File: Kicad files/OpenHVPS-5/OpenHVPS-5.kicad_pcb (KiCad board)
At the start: 2 copper layers, 40.6 x 20.8 mm, 84 parts, among them J1 Conn_01x03_Male, Q1 FQT7N10, Q2 BC846A, Q3 MMBT3906, Q4 MMBT3906, U1 MAX6008AEUR+T, U2 74HC14, U3 MAX4162, U4 CD14538BM

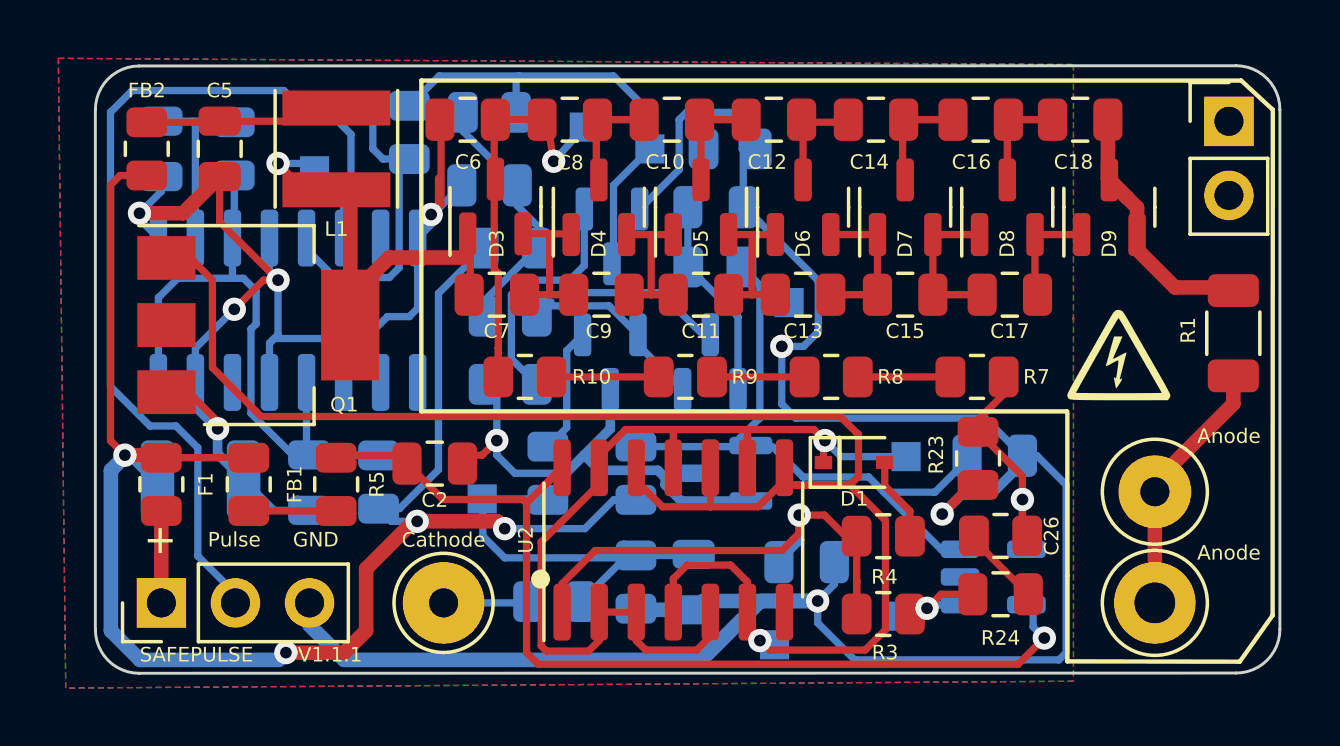
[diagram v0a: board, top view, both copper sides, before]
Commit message: Updated  with TP and some other small changes.
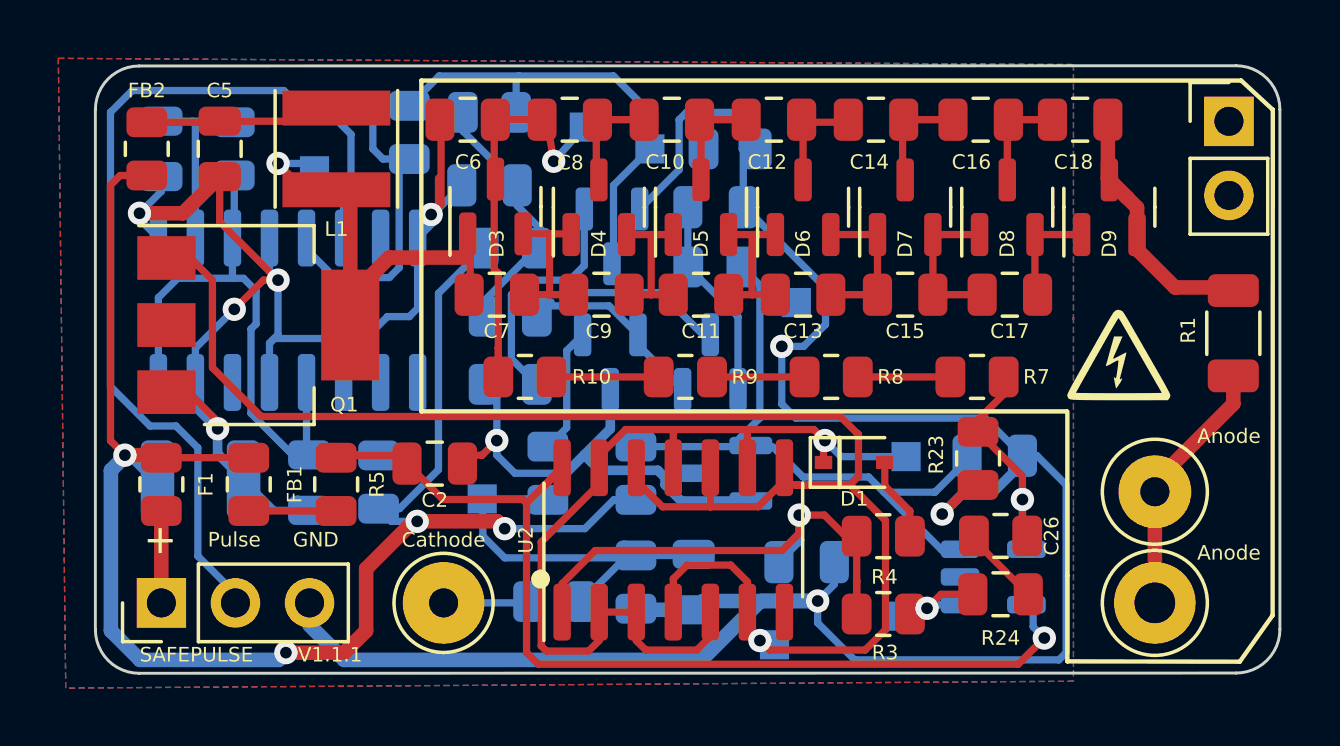
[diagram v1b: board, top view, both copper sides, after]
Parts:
- moved TP1 0.25 mm to (150.3, 65.3)
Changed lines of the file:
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@@
   )
   (footprint "TestPoint:TestPoint_Pad_1.0x1.0mm" (layer "B.Cu")
-    (at 150.02 65.27 180)
+    (at 150.27 65.27 180)
     (descr "SMD rectangular pad as test Point, square 1.0mm side length")
     (tags "test point SMD pad rectangle square")
@@
   (segment (start 142.433 71.12) (end 140.62 71.12) (width 0.25) (layer "B.Cu") (net 3))
   (segment (start 127.75 62.208) (end 127.75 62.41) (width 0.25) (layer "B.Cu") (net 3))
+  (segment (start 148.45 62) (end 148.5 62) (width 0.25) (layer "B.Cu") (net 3))
   (segment (start 152.27 77.52) (end 159.27 77.52) (width 0.25) (layer "B.Cu") (net 3))
-  (segment (start 148.45 62) (end 148.5 62) (width 0.25) (layer "B.Cu") (net 3))
   (segment (start 134.1026 66.5) (end 134.747 67.1444) (width 0.25) (layer "B.Cu") (net 3))
   (segment (start 127.75 62.41) (end 128.397 63.057) (width 0.25) (layer "B.Cu") (net 3))
   (segment (start 139.428 68.072) (end 139.5495 68.072) (width 0.25) (layer "B.Cu") (net 3))
+  (segment (start 151.27 64.77) (end 151.27 66.02) (width 0.25) (layer "B.Cu") (net 3))
   (segment (start 137.832 62.332) (end 137.832 62.5121) (width 0.25) (layer "B.Cu") (net 3))
   (segment (start 149.77 68.75) (end 150.25 69.23) (width 0.25) (layer "B.Cu") (net 3))
@@
   (segment (start 137.75 62.25) (end 137.8 62.25) (width 0.25) (layer "B.Cu") (net 3))
   (segment (start 151 76.25) (end 152.27 77.52) (width 0.25) (layer "B.Cu") (net 3))
+  (segment (start 150.52 66.77) (end 149.77 66.77) (width 0.25) (layer "B.Cu") (net 3))
   (segment (start 148.4125 59.1625) (end 148.4125 60) (width 0.25) (layer "B.Cu") (net 3))
   (segment (start 149.04 75.5) (end 151 75.5) (width 0.5) (layer "B.Cu") (net 3))
@@
   (segment (start 148.336 72.0325) (end 148.37 72.0665) (width 0.25) (layer "B.Cu") (net 3))
   (segment (start 158.02 70.77) (end 158.02 70.52) (width 0.3302) (layer "B.Cu") (net 3))
-  (segment (start 151.02 64.52) (end 151.02 66.27) (width 0.25) (layer "B.Cu") (net 3))
   (segment (start 132.5 64.5) (end 132.5 66.3677) (width 0.25) (layer "B.Cu") (net 3))
   (segment (start 151 75.5) (end 151 76.25) (width 0.25) (layer "B.Cu") (net 3))
@@
   (segment (start 128.5 61.458) (end 128.5 60.95) (width 0.25) (layer "B.Cu") (net 3))
   (segment (start 142.993864 70.493864) (end 143.52 71.02) (width 0.3302) (layer "B.Cu") (net 3))
-  (segment (start 150.52 66.77) (end 149.77 66.77) (width 0.25) (layer "B.Cu") (net 3))
   (segment (start 159.27 77.52) (end 159.52 77.27) (width 0.25) (layer "B.Cu") (net 3))
   (segment (start 149.77 66.77) (end 149.77 68.75) (width 0.25) (layer "B.Cu") (net 3))
@@
   (segment (start 143.891 69.596728) (end 142.993864 70.493864) (width 0.3302) (layer "B.Cu") (net 3))
   (segment (start 140.62 71.12) (end 140 70.5) (width 0.25) (layer "B.Cu") (net 3))
+  (segment (start 151.27 66.02) (end 150.52 66.77) (width 0.25) (layer "B.Cu") (net 3))
   (segment (start 132.207 66.6607) (end 132.3677 66.5) (width 0.25) (layer "B.Cu") (net 3))
   (segment (start 143.891 68.2475) (end 143.891 69.596728) (width 0.3302) (layer "B.Cu") (net 3))
@@
   (segment (start 133.4615 72.5) (end 133.57 72.3915) (width 0.25) (layer "B.Cu") (net 3))
   (segment (start 132.5 64.5) (end 132.207 64.207) (width 0.25) (layer "B.Cu") (net 3))
-  (segment (start 148.5 62) (end 151.02 64.52) (width 0.25) (layer "B.Cu") (net 3))
   (segment (start 158.52 70.52) (end 158.02 70.52) (width 0.25) (layer "B.Cu") (net 3))
   (segment (start 137 65.75) (end 137.287 65.463) (width 0.25) (layer "B.Cu") (net 3))
@@
   (segment (start 157.02 71.77) (end 158.02 70.77) (width 0.3302) (layer "B.Cu") (net 3))
   (segment (start 151.5 74.096) (end 151.572 74.168) (width 0.25) (layer "B.Cu") (net 3))
-  (segment (start 151.02 66.27) (end 150.52 66.77) (width 0.25) (layer "B.Cu") (net 3))
   (segment (start 130.429 70.4525) (end 131.318 71.3415) (width 0.3302) (layer "B.Cu") (net 3))
   (segment (start 129.667 66.833) (end 129.667 68.007) (width 0.25) (layer "B.Cu") (net 3))
   (segment (start 140 70) (end 140 68.5225) (width 0.25) (layer "B.Cu") (net 3))
   (segment (start 148.45 62) (end 148.45 60.0375) (width 0.25) (layer "B.Cu") (net 3))
+  (segment (start 148.5 62) (end 151.27 64.77) (width 0.25) (layer "B.Cu") (net 3))
   (segment (start 146.32 72.07) (end 148.7075 72.07) (width 0.3302) (layer "B.Cu") (net 3))
   (segment (start 134.05 59.05) (end 134.5 58.6) (width 0.25) (layer "F.Cu") (net 4))
